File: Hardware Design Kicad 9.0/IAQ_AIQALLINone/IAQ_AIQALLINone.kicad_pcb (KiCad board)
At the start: 2 copper layers, 5 parts, among them IC1 ENS160-BGLT, IC2 SGP41-D-R4, U1 RASPBERRY_PI_4B_4GB, U3 BME688

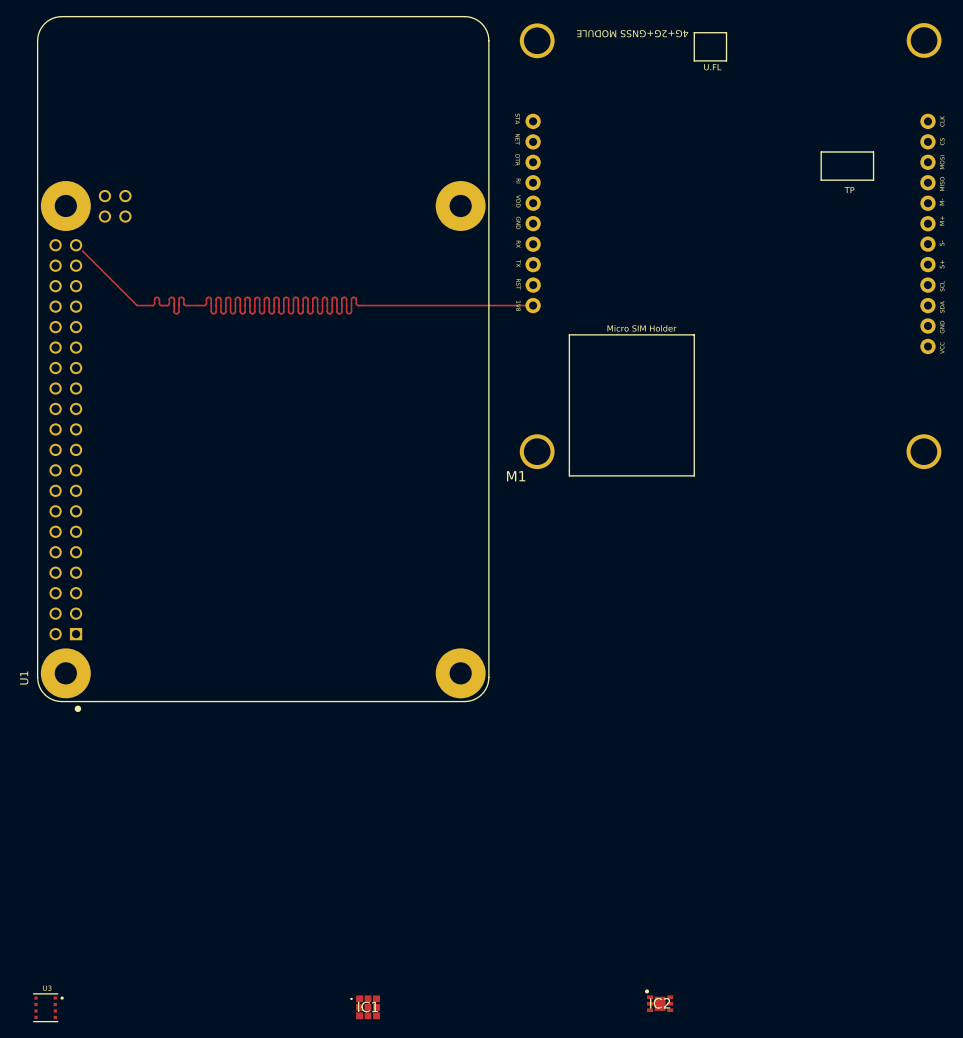
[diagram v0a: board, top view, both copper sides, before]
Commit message: update
141619032026
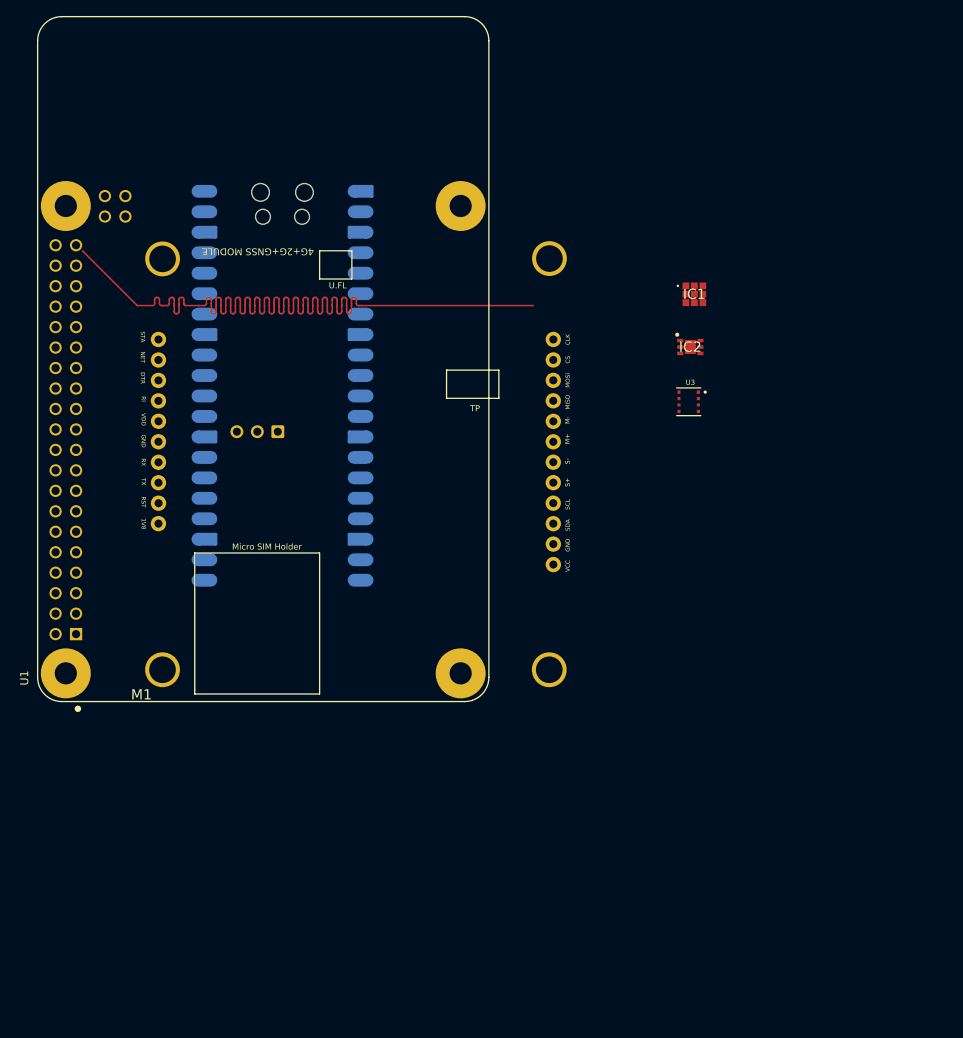
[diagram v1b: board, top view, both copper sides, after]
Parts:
- added U2: RASPBERRY_PI_PICO_W, Module:RaspberryPi_Pico_W_SMD_HandSolder, B.Cu at (104.9, 88.3)
- moved U3 109.6 mm to (155.3, 90.3)
- moved IC1 97.3 mm to (156.0, 77.0)
- moved IC2 81.6 mm to (155.5, 83.5)
- moved M1 53.8 mm to (87.4, 126.7)
